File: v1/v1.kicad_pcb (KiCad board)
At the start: 2 copper layers, 82 x 91.2 mm, 7 parts, among them J1 Conn_02x22_Top_Bottom, U1 ESP32-S3-DevKitC, U2 DM-OLED096-636

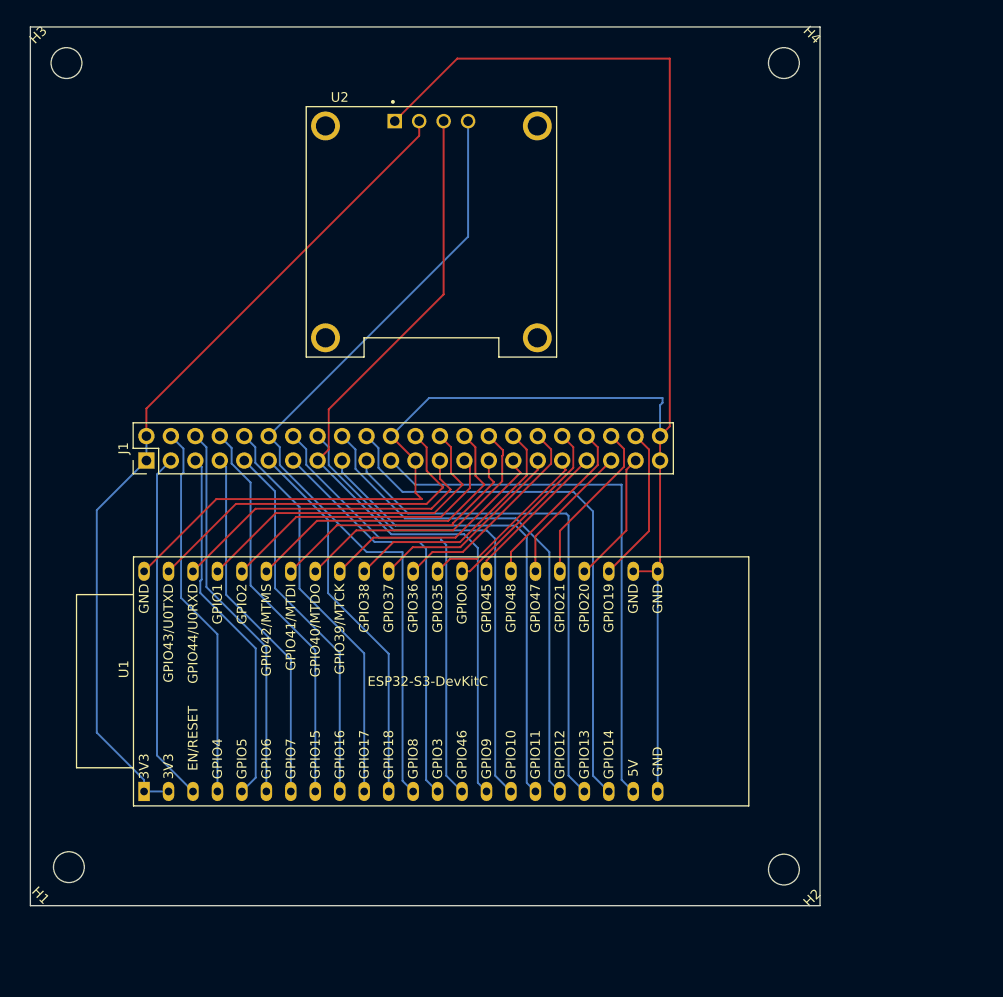
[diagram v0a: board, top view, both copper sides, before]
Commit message: code, new pcb and bom
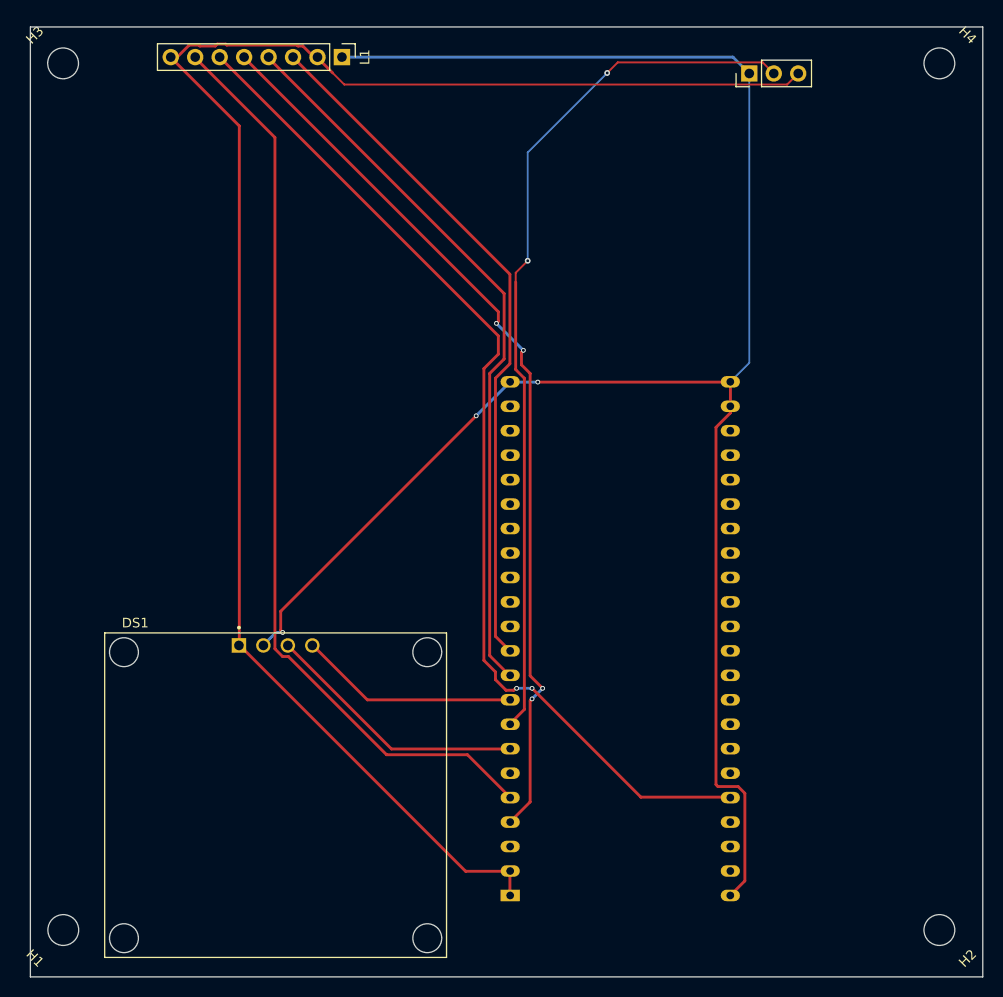
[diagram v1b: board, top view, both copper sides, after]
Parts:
- removed J1: Conn_02x22_Top_Bottom, Connector_PinHeader_2.54mm:PinHeader_2x22_P2.54mm_Vertical
- removed U2: DM-OLED096-636, Library:MODULE_DM-OLED096-636
- added DS1: OLED_128X64_1.3_I2C, LCD_OLED_128X64_1.3_I2C:LCD_OLED_128X64_1.3_I2C, F.Cu at (122.1, 108.0)
- added L1: ~, Connector_PinHeader_2.54mm:PinHeader_1x08_P2.54mm_Vertical, F.Cu at (129.0, 31.4)
- added T1: ~, Connector_PinHeader_2.54mm:PinHeader_1x03_P2.54mm_Vertical, F.Cu at (171.3, 33.0)
- U1: moved to B.Cu
- moved U1 39.5 mm to (146.4, 118.4), turned to 0 degrees
- moved H2 17.3 mm to (191.0, 122.0)
- moved H4 16.1 mm to (191.0, 32.0)
- moved H1 6.55 mm to (100.0, 122.0)
- moved H3 0.35 mm to (100.0, 32.0)
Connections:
- U1 pad 12: Net-(J1-Pin_12) -> unconnected-(U1-GPIO8/ADC1_CH7-Pad12)
- U1 pad 13: Net-(J1-Pin_13) -> unconnected-(U1-GPIO3/ADC1_CH2-Pad13)
- U1 pad 14: Net-(J1-Pin_14) -> unconnected-(U1-GPIO46-Pad14)
- U1 pad 15: Net-(J1-Pin_15) -> unconnected-(U1-GPIO9/ADC1_CH8-Pad15)
- U1 pad 16: Net-(J1-Pin_16) -> unconnected-(U1-GPIO10/ADC1_CH9-Pad16)
- U1 pad 17: Net-(J1-Pin_17) -> unconnected-(U1-GPIO11/ADC2_CH0-Pad17)
- U1 pad 18: Net-(J1-Pin_18) -> unconnected-(U1-GPIO12/ADC2_CH1-Pad18)
- U1 pad 19: Net-(J1-Pin_19) -> unconnected-(U1-GPIO13/ADC2_CH2-Pad19)
- U1 pad 20: Net-(J1-Pin_20) -> unconnected-(U1-GPIO14/ADC2_CH3-Pad20)
- U1 pad 21: Net-(J1-Pin_21) -> unconnected-(U1-5V-Pad21)
- U1 pad 25: Net-(J1-Pin_42) -> unconnected-(U1-GPIO19/USB_D--Pad25)
- U1 pad 26: Net-(J1-Pin_41) -> unconnected-(U1-GPIO20/USB_D+-Pad26)
- U1 pad 27: Net-(J1-Pin_40) -> unconnected-(U1-GPIO21-Pad27)
- U1 pad 28: Net-(J1-Pin_39) -> unconnected-(U1-GPIO47-Pad28)
- U1 pad 29: Net-(J1-Pin_38) -> unconnected-(U1-GPIO48-Pad29)
- U1 pad 3: Net-(J1-Pin_3) -> unconnected-(U1-CHIP_PU-Pad3)
- U1 pad 30: Net-(J1-Pin_37) -> unconnected-(U1-GPIO45-Pad30)
- U1 pad 31: Net-(J1-Pin_36) -> unconnected-(U1-GPIO0-Pad31)
- U1 pad 32: Net-(J1-Pin_35) -> unconnected-(U1-GPIO35-Pad32)
- U1 pad 33: Net-(J1-Pin_34) -> unconnected-(U1-GPIO36-Pad33)
- U1 pad 34: Net-(J1-Pin_33) -> unconnected-(U1-GPIO37-Pad34)
- U1 pad 35: Net-(J1-Pin_32) -> unconnected-(U1-GPIO38-Pad35)
- U1 pad 36: Net-(J1-Pin_31) -> unconnected-(U1-GPIO39/MTCK-Pad36)
- U1 pad 37: Net-(J1-Pin_30) -> unconnected-(U1-GPIO40/MTDO-Pad37)
- U1 pad 38: Net-(J1-Pin_29) -> unconnected-(U1-GPIO41/MTDI-Pad38)
- U1 pad 39: Net-(J1-Pin_28) -> unconnected-(U1-GPIO42/MTMS-Pad39)
- U1 pad 41: Net-(J1-Pin_26) -> unconnected-(U1-GPIO1/ADC1_CH0-Pad41)
- U1 pad 42: Net-(J1-Pin_25) -> unconnected-(U1-GPIO44/U0RXD-Pad42)
- U1 pad 43: Net-(J1-Pin_24) -> unconnected-(U1-GPIO43/U0TXD-Pad43)
- U1 pad 6: Net-(J1-Pin_6) -> unconnected-(U1-GPIO6/ADC1_CH5-Pad6)
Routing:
- net Net-(J1-Pin_15): track 86.7 -> 0.00 mm
- net Net-(J1-Pin_12): track 86.6 -> 0.00 mm
- net Net-(DS1-VDD): track 88.1 -> 172.4 mm
- net Net-(L1-DC): track 30.4 -> 107.4 mm, vias 0 -> 2
- net Net-(L1-BL): track 37.7 -> 95.7 mm
- net Net-(J1-Pin_20): track 57.7 -> 0.00 mm
- net Net-(J1-Pin_21): track 57.3 -> 0.00 mm
- net Net-(L1-RES): track 39.1 -> 94.1 mm, vias 0 -> 4
- net Net-(J1-Pin_19): track 53.4 -> 0.00 mm
- net Net-(J1-Pin_18): track 53.0 -> 0.00 mm
- net Net-(J1-Pin_16): track 50.9 -> 0.00 mm
- net Net-(J1-Pin_17): track 50.0 -> 0.00 mm
- net Net-(T1-IO): track 41.0 -> 90.8 mm, vias 0 -> 2
- net Net-(J1-Pin_14): track 47.9 -> 0.00 mm
- net Net-(J1-Pin_13): track 43.3 -> 0.00 mm
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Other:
- board size 82 x 91.2 mm -> 98.9 x 98.6 mm

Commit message: new PCB schematic, readme, BOM
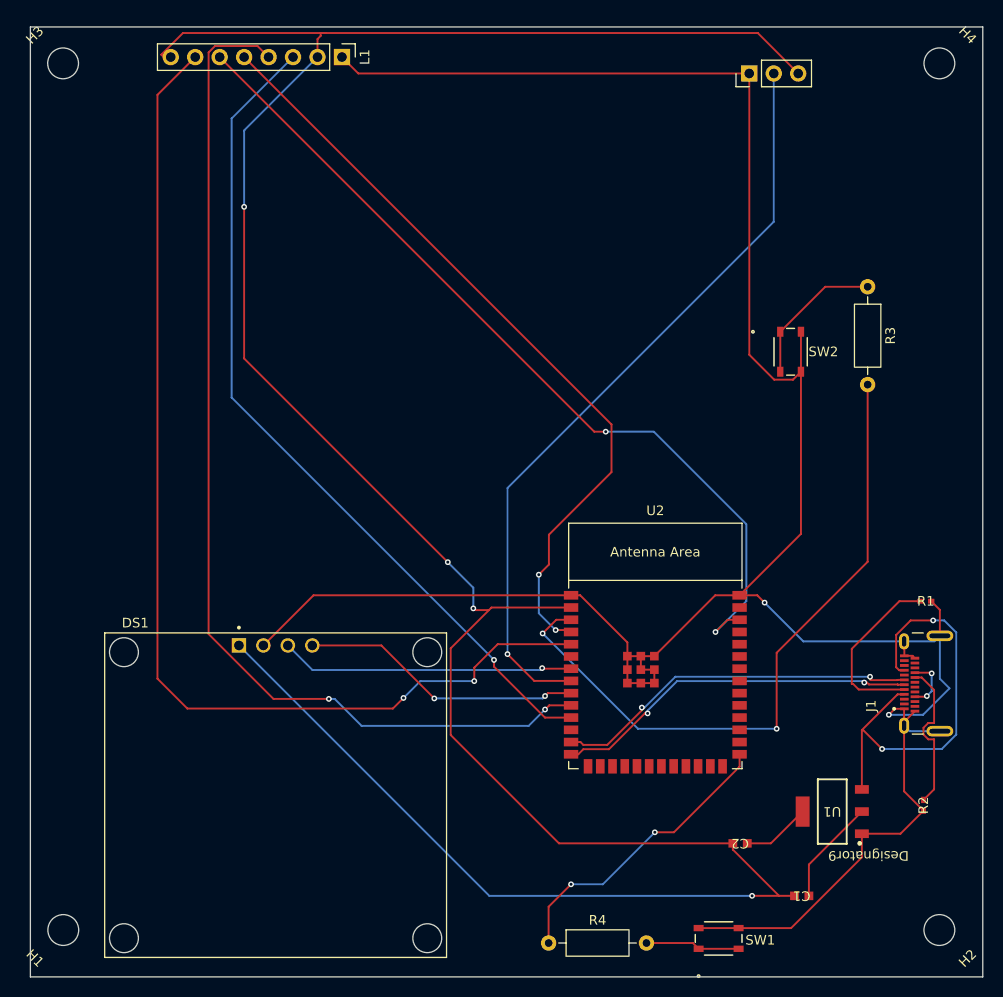
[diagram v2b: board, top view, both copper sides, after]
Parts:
- added C1: GRM188R60J106KE47D, footprints:CAP_GRM188_1608_MUR, F.Cu at (176.7, 118.5)
- added C2: GRM188R60J106KE47D, footprints:CAP_GRM188_1608_MUR, F.Cu at (170.3, 113.0)
- added J1: CX90BW1-24P1, footprints:HIROSE_CX90BW1-24P1, F.Cu at (191.1, 96.4)
- added R1: RC0402FR-075K1L, footprints:RC0402N_YAG, F.Cu at (189.6, 87.8)
- added R2: RC0402FR-075K1L, footprints:RC0402N_YAG, F.Cu at (189.3, 109.0)
- added R3: 10k, Resistor_THT:R_Axial_DIN0207_L6.3mm_D2.5mm_P10.16mm_Horizontal, F.Cu at (183.6, 55.2)
- added R4: 10k, Resistor_THT:R_Axial_DIN0207_L6.3mm_D2.5mm_P10.16mm_Horizontal, F.Cu at (150.4, 123.3)
- added SW1: SKRPABE010, footprints:SW4_SKRPABE010_ALPS, F.Cu at (168.1, 122.9)
- added SW2: SKRPABE010, footprints:SW4_SKRPABE010_ALPS, F.Cu at (175.6, 62.0)
- added U2: ESP32-S3-WROOM-1, PCM_Espressif:ESP32-S3-WROOM-1, F.Cu at (161.5, 95.5)
- U1: value ESP32-S3-DevKitC -> TLV1117-33IDCYR; footprint PCM_Espressif:ESP32-S3-DevKitC -> footprints:DCY0004A_L; moved to F.Cu
- moved U1 34.6 mm to (179.9, 109.7), turned to 180 degrees
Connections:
- DS1 pad 1: Net-(DS1-VDD) -> 3V3
- DS1 pad 2: Net-(DS1-GND) -> GND
- DS1 pad 3: Net-(DS1-SCK) -> GPIO7
- DS1 pad 4: Net-(DS1-SDA) -> GPIO16
- L1 pad 1: Net-(DS1-GND) -> GND
- L1 pad 2: Net-(DS1-VDD) -> 3V3
- L1 pad 3: Net-(L1-SCL) -> GPIO18
- L1 pad 4: Net-(L1-SDA) -> GPIO17
- L1 pad 5: Net-(L1-RES) -> GPIO4
- L1 pad 6: Net-(L1-DC) -> GPIO2
- L1 pad 7: Net-(L1-BL) -> GPIO5
- L1 pad 8: Net-(DS1-VDD) -> 3V3
- T1 pad 1: Net-(DS1-GND) -> GND
- T1 pad 2: Net-(T1-IO) -> GPIO15
- T1 pad 3: Net-(DS1-VDD) -> 3V3
- U1 pad 1: Net-(DS1-VDD) -> GND
- U1 pad 2: Net-(DS1-VDD) -> Net-(C1-Pad1)
- U1 pad 3: unconnected-(U1-CHIP_PU-Pad3) -> VBUS
- U1 pad 4: Net-(L1-RES) -> Net-(C2-Pad1)
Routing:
- net 3V3: track 0.00 -> 278.3 mm, vias 0 -> 4
- net GND: track 0.00 -> 268.7 mm, vias 0 -> 2
- net Net-(DS1-GND): track 194.5 -> 0.00 mm, vias 3 -> 0
- net Net-(DS1-VDD): track 172.4 -> 0.00 mm
- net GPIO5: track 0.00 -> 114.0 mm, vias 0 -> 2
- net GPIO17: track 0.00 -> 109.9 mm, vias 0 -> 2
- net Net-(L1-DC): track 107.4 -> 0.00 mm, vias 2 -> 0
- net Net-(L1-BL): track 95.7 -> 0.00 mm
- net Net-(L1-RES): track 94.1 -> 0.00 mm, vias 4 -> 0
- net Net-(T1-IO): track 90.8 -> 0.00 mm, vias 2 -> 0
- net GPIO2: track 0.00 -> 90.3 mm, vias 0 -> 2
- net GPIO18: track 0.00 -> 87.4 mm, vias 0 -> 1
- net GPIO4: track 0.00 -> 80.8 mm, vias 0 -> 2
- net GPIO15: track 0.00 -> 79.5 mm, vias 0 -> 1
- net Net-(L1-SDA): track 76.0 -> 0.00 mm
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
